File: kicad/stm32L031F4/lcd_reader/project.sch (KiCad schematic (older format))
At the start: 33 parts, among them J1 WAKE, J10 TEST_1P, J11 TEST_1P, J12 TEST_1P, J13 GND_EXT, J2 SWD, J3 TEST_1P, J4 TEST_1P, J5 TEST_1P, J6 LCD, J7 TEST_1P, J8 RADIO, J9 TEST_1P, Q1 CSD16414Q5, U1 74LS14, U2 STM32L031F4Px, U3 74LS14

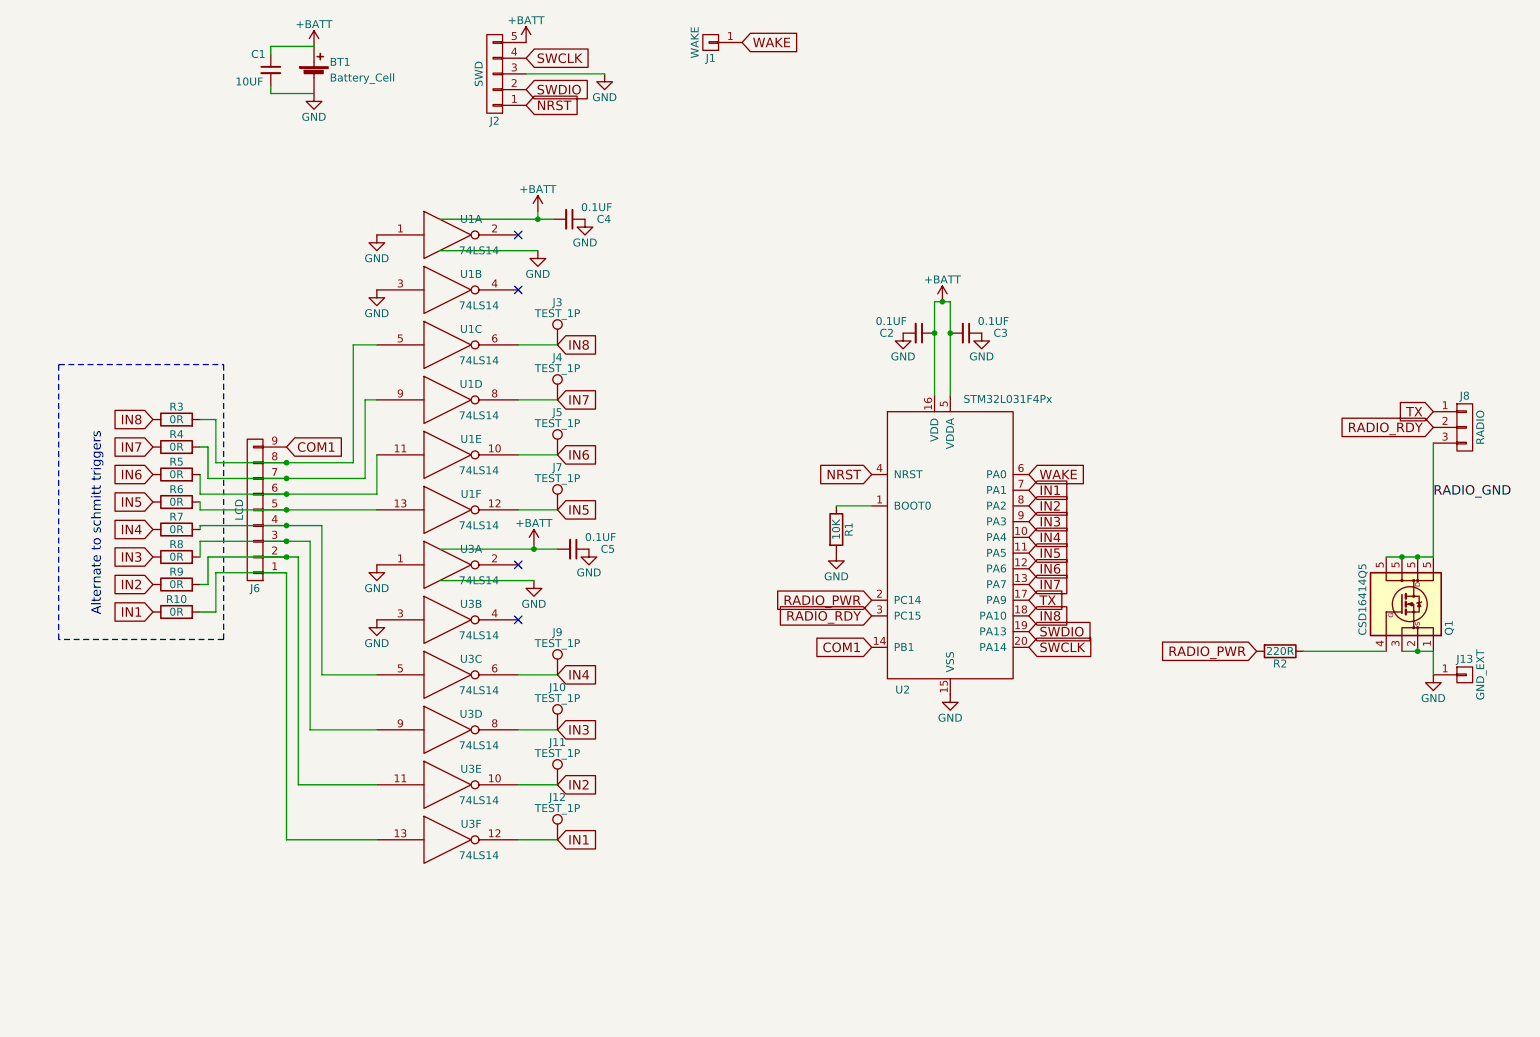
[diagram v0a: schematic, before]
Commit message: Silkscreen tidying
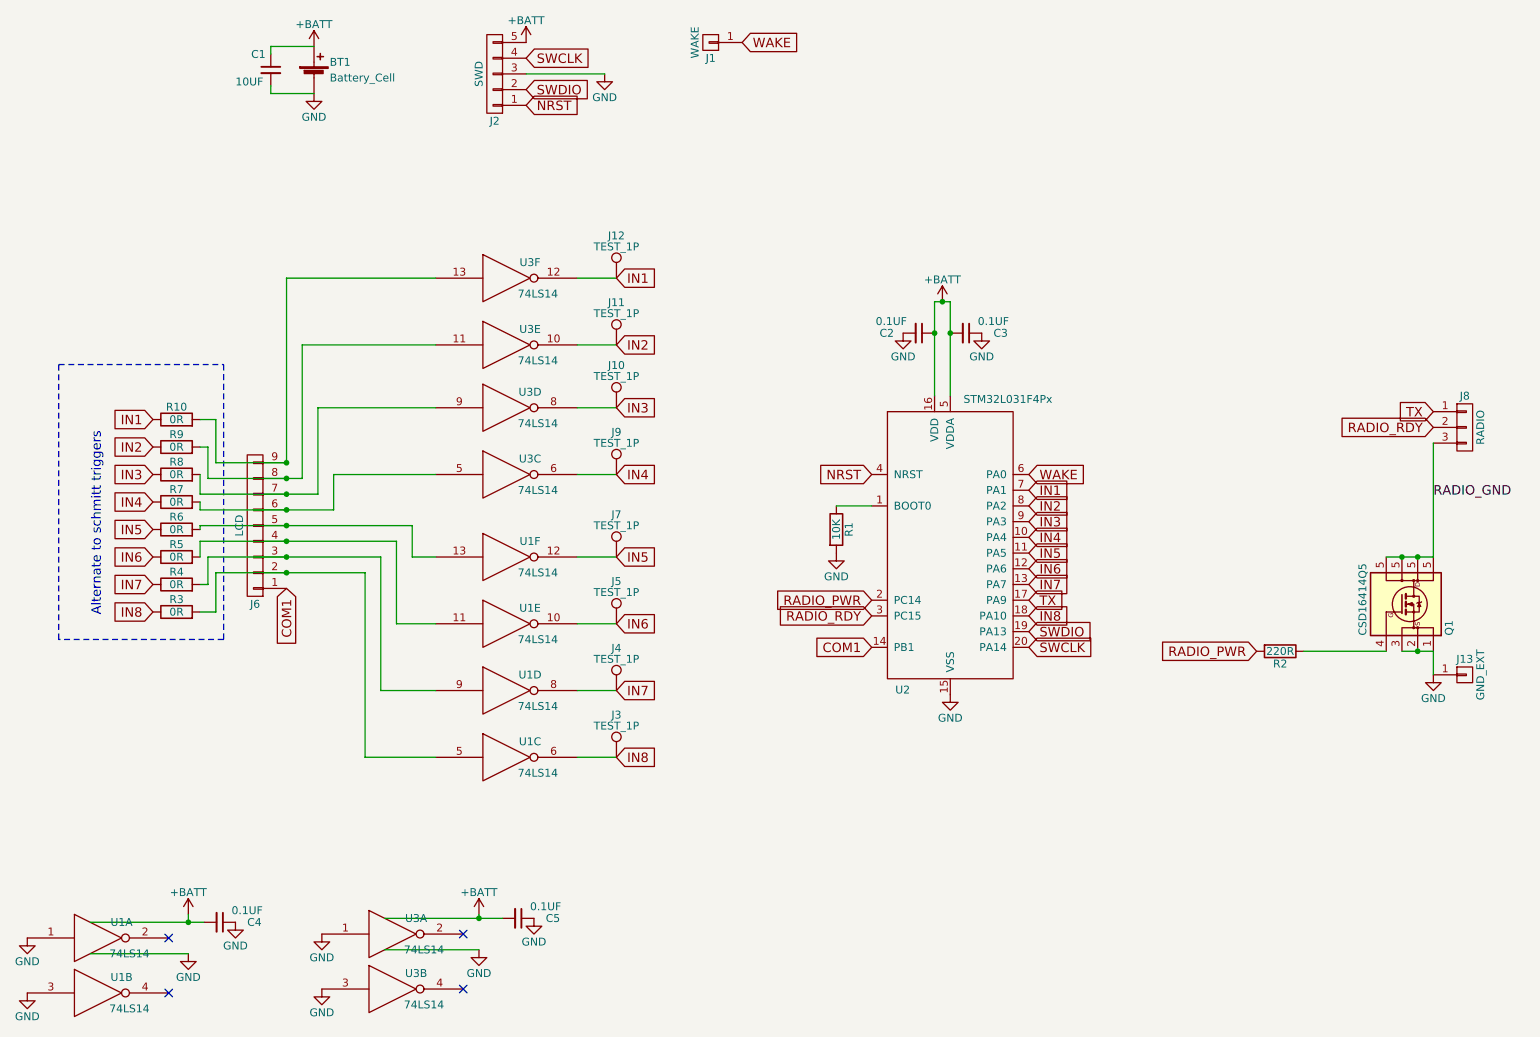
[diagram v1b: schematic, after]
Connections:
- net COM1: now also J6.1 (P1); no longer J6.9 (P9)
- net at R10.2, U3.13: now also J6.9 (P9); no longer J6.1 (P1)
- net at R9.2, U3.11: now also J6.8 (P8); no longer J6.2 (P2)
- net at R8.2, U3.9: now also J6.7 (P7); no longer J6.3 (P3)
- net at R7.2, U3.5: now also J6.6 (P6); no longer J6.4 (P4)
- net at R5.2, U1.11: now also J6.4 (P4); no longer J6.6 (P6)
- net at R4.2, U1.9: now also J6.3 (P3); no longer J6.7 (P7)
- net at R3.2, U1.5: now also J6.2 (P2); no longer J6.8 (P8)
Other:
- moved on the sheet: C4, C5, J10, J11, J12, J3, J4, J5, J6, J7, J9, R10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
